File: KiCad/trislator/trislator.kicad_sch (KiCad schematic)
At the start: 18 parts, among them J1 Conn_01x02, J2 Conn_01x02, J3 Conn_01x03, J4 Conn_01x03, U1 D168K, U10 D168K, U11 D168K, U12 74HC595, U13 74HC595, U14 74HC595, U2 D168K, U3 D168K, U4 D168K, U5 D168K, U6 D168K, U7 D168K, U8 D168K, U9 D168K

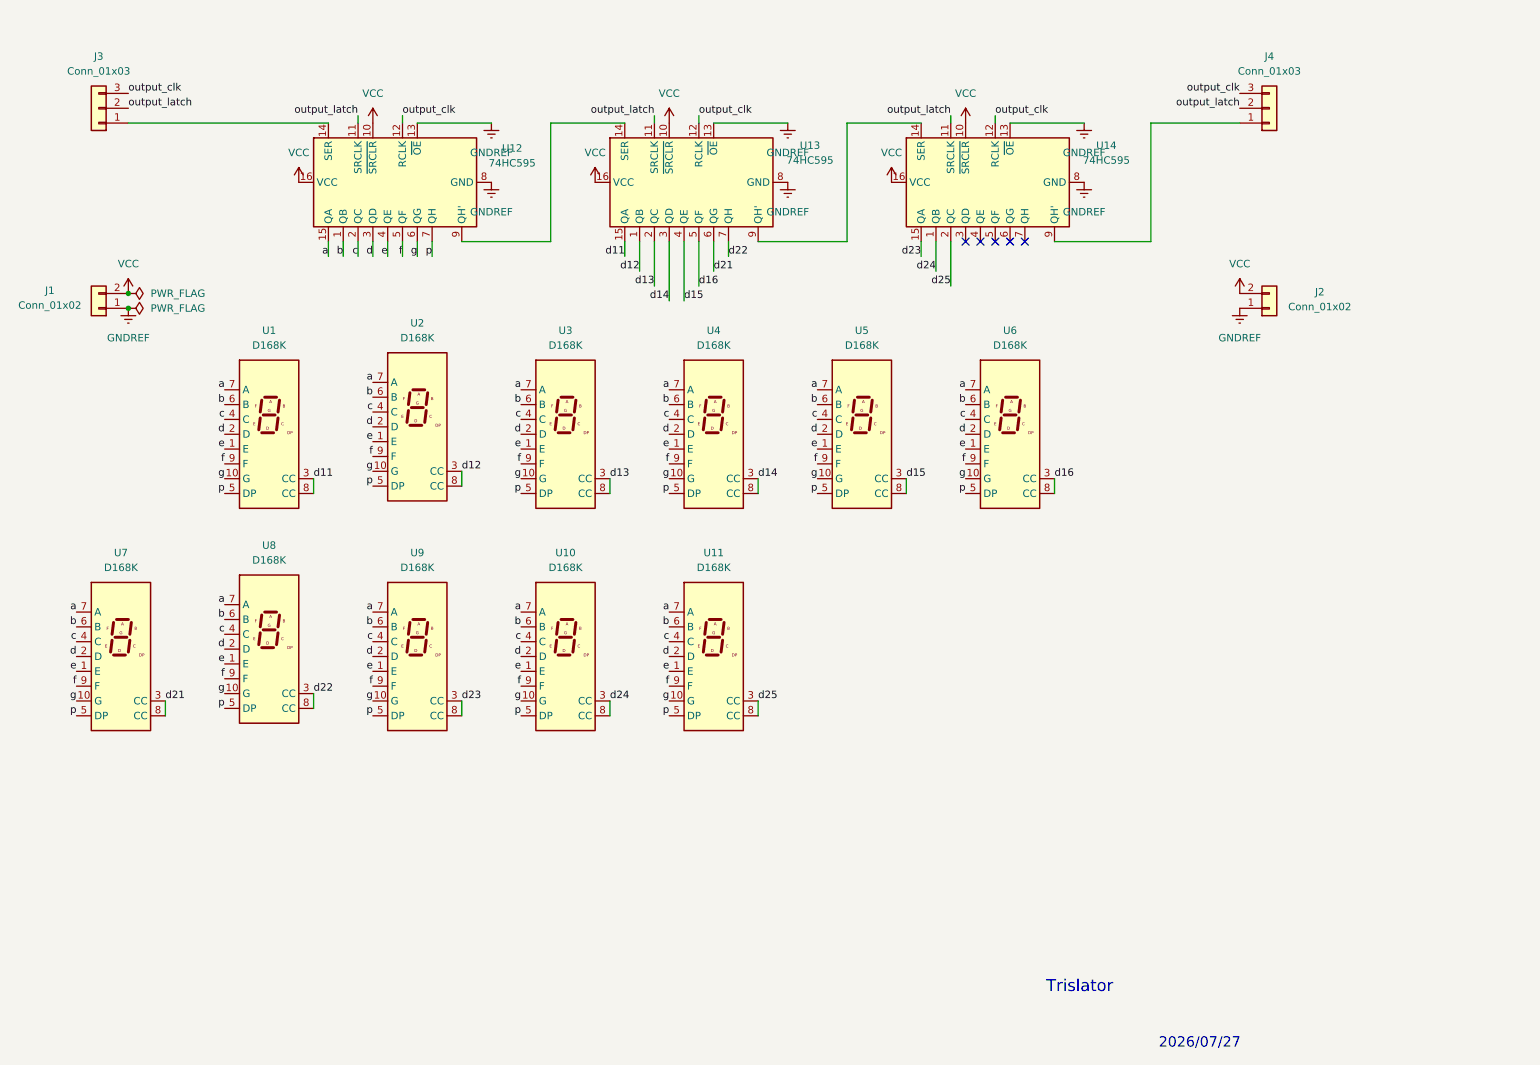
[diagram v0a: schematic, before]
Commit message: finish trislator schematic
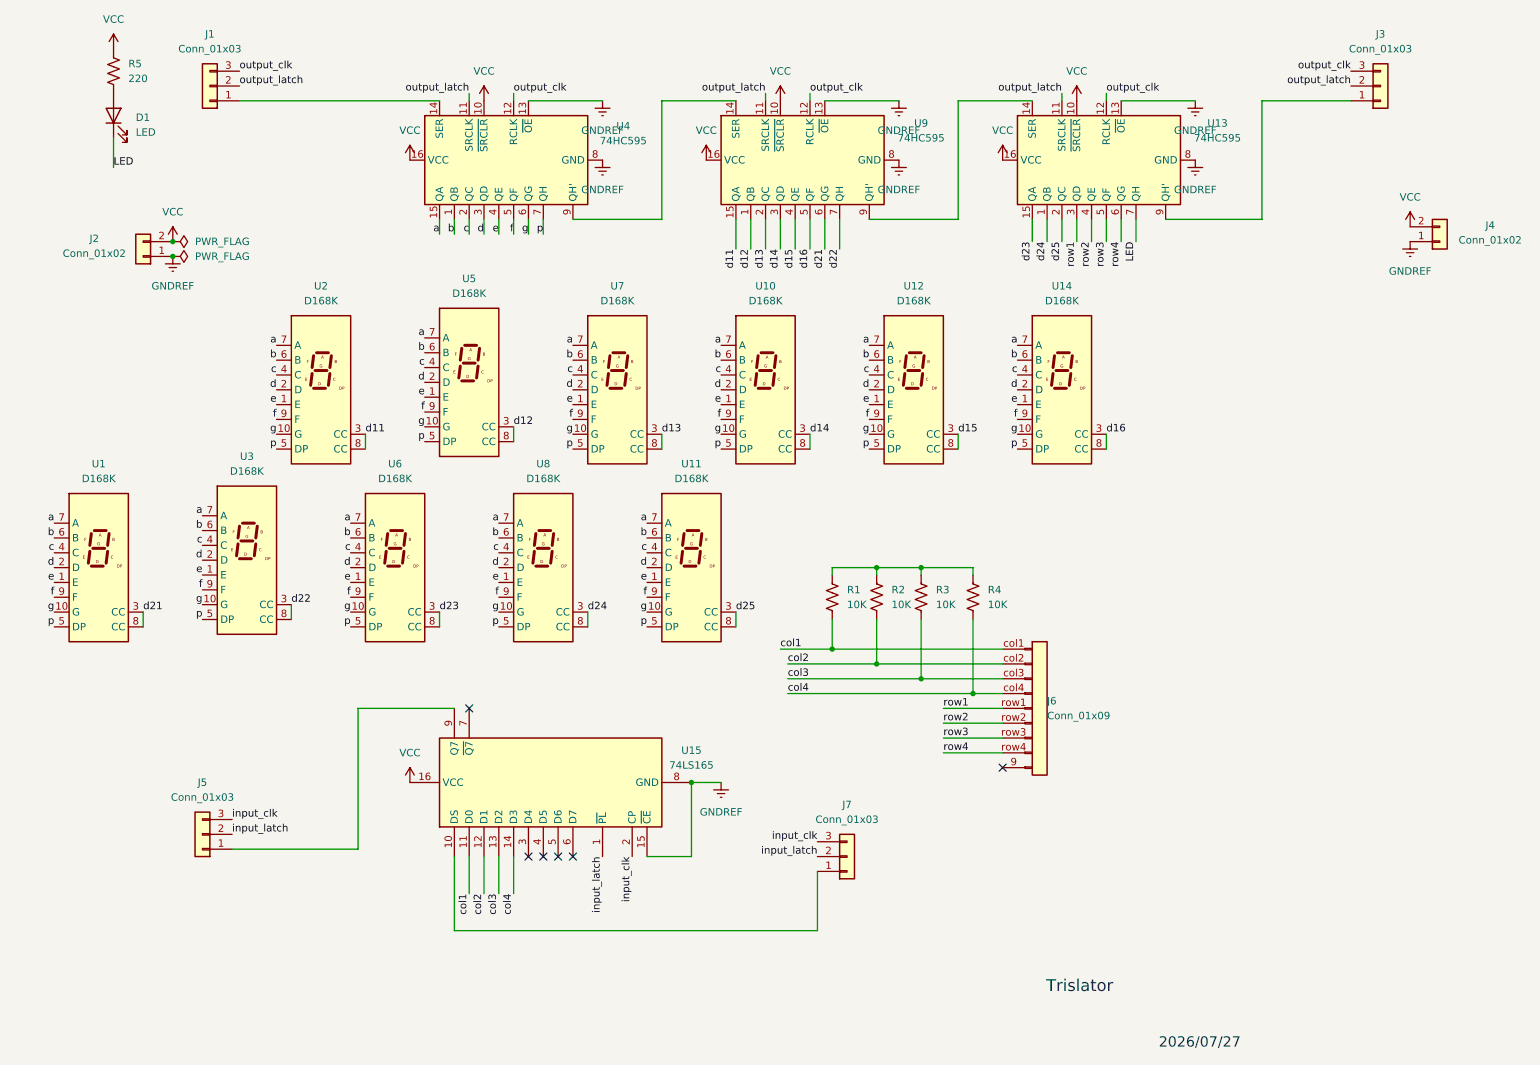
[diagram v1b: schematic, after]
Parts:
- removed J1: Conn_01x02, symbol Connector_Generic:Conn_01x02
- removed J4: Conn_01x03, symbol Connector_Generic:Conn_01x03
- removed U12, U14: 74HC595, symbol 74xx:74HC595
- removed U4, U9: D168K, Display_7Segment:D1X8K, symbol Display_Character:D168K
- added D1: LED, symbol Device:LED
- added J1, J5, J7: Conn_01x03, Connector_PinHeader_2.54mm:PinHeader_1x03_P2.54mm_Horizontal, symbol Connector_Generic:Conn_01x03
- added J4: Conn_01x02, Connector_PinHeader_2.54mm:PinHeader_1x02_P2.54mm_Horizontal, symbol Connector_Generic:Conn_01x02
- added J6: Conn_01x09, symbol Connector_Generic:Conn_01x09
- added R1, R2, R3, R4: 10K, symbol Device:R_US
- added R5: 220, symbol Device:R_US
- added U12, U14: D168K, Display_7Segment:D1X8K, symbol Display_Character:D168K
- added U15: 74LS165, symbol 74xx:74LS165
- added U4, U9: 74HC595, Package_DIP:DIP-16_W7.62mm, symbol 74xx:74HC595
- J2: footprint (none) -> Connector_PinHeader_2.54mm:PinHeader_1x02_P2.54mm_Horizontal
- J3: footprint (none) -> Connector_PinHeader_2.54mm:PinHeader_1x03_P2.54mm_Horizontal
- U13: footprint (none) -> Package_DIP:DIP-16_W7.62mm
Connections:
- net GNDREF: now also J4.1 (Pin_1), U15.15 (~{CE}), U15.8 (GND), U4.13 (~{OE}), U4.8 (GND), U9.13 (~{OE}), U9.8 (GND)
- net VCC: now also J4.2 (Pin_2), R5.1, U15.16 (VCC), U4.10 (~{SRCLR}), U4.16 (VCC), U9.10 (~{SRCLR}), U9.16 (VCC)
- net a: now also U12.7 (A), U14.7 (A), U4.15 (QA)
- net b: now also U12.6 (B), U14.6 (B), U4.1 (QB)
- net c: now also U12.4 (C), U14.4 (C), U4.2 (QC)
- net d: now also U12.2 (D), U14.2 (D), U4.3 (QD)
- net d11: now also U2.3 (CC), U2.8 (CC), U9.15 (QA); no longer U1.3 (CC), U1.8 (CC), U13.15 (QA)
- net d12: now also U5.3 (CC), U5.8 (CC), U9.1 (QB); no longer U13.1 (QB), U2.3 (CC), U2.8 (CC)
- net d13: now also U7.3 (CC), U7.8 (CC), U9.2 (QC); no longer U13.2 (QC), U3.3 (CC), U3.8 (CC)
- net d14: now also U10.3 (CC), U10.8 (CC), U9.3 (QD); no longer U13.3 (QD)
- net d15: now also U12.3 (CC), U12.8 (CC), U9.4 (QE); no longer U13.4 (QE), U5.3 (CC), U5.8 (CC)
- net d16: now also U14.3 (CC), U14.8 (CC), U9.5 (QF); no longer U13.5 (QF), U6.3 (CC), U6.8 (CC)
- net d21: now also U1.3 (CC), U1.8 (CC), U9.6 (QG); no longer U13.6 (QG), U7.3 (CC), U7.8 (CC)
- net d22: now also U3.3 (CC), U3.8 (CC), U9.7 (QH); no longer U13.7 (QH), U8.3 (CC), U8.8 (CC)
- net d23: now also U13.15 (QA), U6.3 (CC), U6.8 (CC)
- net d24: now also U13.1 (QB), U8.3 (CC), U8.8 (CC); no longer U10.3 (CC), U10.8 (CC)
- net d25: now also U13.2 (QC)
- net e: now also U12.1 (E), U14.1 (E), U4.4 (QE)
- net f: now also U12.9 (F), U14.9 (F), U4.5 (QF)
- net g: now also U12.10 (G), U14.10 (G), U4.6 (QG)
- net output_clk: now also J1.3 (Pin_3), U4.12 (RCLK), U9.12 (RCLK)
- net output_latch: now also J1.2 (Pin_2), U4.11 (SRCLK), U9.11 (SRCLK)
- net p: now also U12.5 (DP), U14.5 (DP), U4.7 (QH)
- net at J3.1 (Pin_1): now also U13.9 (QH')
- net at U13.14 (SER): now also U9.9 (QH')
- new net: J1.1 (Pin_1), U4.14 (SER)
- new net: U4.9 (QH'), U9.14 (SER)
- new net: D1.2 (A), R5.2
- new net: J7.1 (Pin_1), U15.10 (DS)
- new net: J5.1 (Pin_1), U15.9 (Q7)
- new net: R1.1, R2.1, R3.1, R4.1
- new net LED: D1.1 (K), U13.7 (QH)
- new net col1: J6.col1 (Pin_1), R1.2, U15.11 (D0)
- new net col2: J6.col2 (Pin_2), R2.2, U15.12 (D1)
- new net col3: J6.col3 (Pin_3), R3.2, U15.13 (D2)
- new net col4: J6.col4 (Pin_4), R4.2, U15.14 (D3)
- new net input_clk: J5.3 (Pin_3), J7.3 (Pin_3), U15.2 (CP)
- new net input_latch: J5.2 (Pin_2), J7.2 (Pin_2), U15.1 (~{PL})
- new net row1: J6.row1 (Pin_5), U13.3 (QD)
- new net row2: J6.row2 (Pin_6), U13.4 (QE)
- new net row3: J6.row3 (Pin_7), U13.5 (QF)
- new net row4: J6.row4 (Pin_8), U13.6 (QG)
- no-connect marks 5 -> 6
